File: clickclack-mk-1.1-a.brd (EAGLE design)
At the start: 101.6 x 25.4 mm, 23 parts, among them SW1 CHERRY-MXNONUBS, SW2 CHERRY-MXNONUBS, SW3 CHERRY-MXNONUBS, SW4 CHERRY-MXNONUBS, SW5 CHERRY-MXNONUBS, SW6 CHERRY-MXNONUBS, U1 TEENSY_3.0_BASIC_ALTDIP

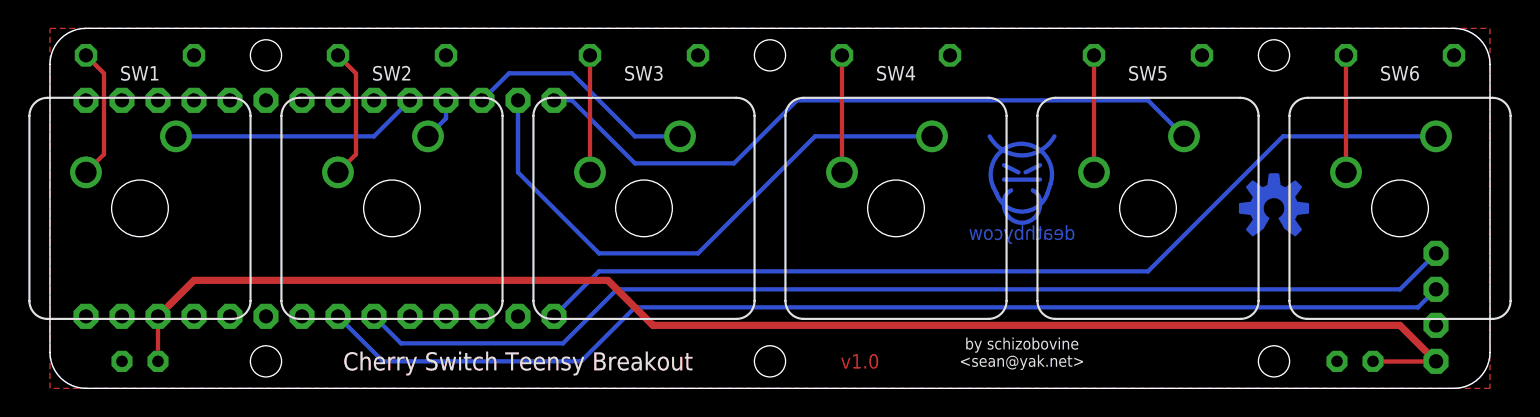
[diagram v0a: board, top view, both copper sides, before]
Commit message: [wip] do not use
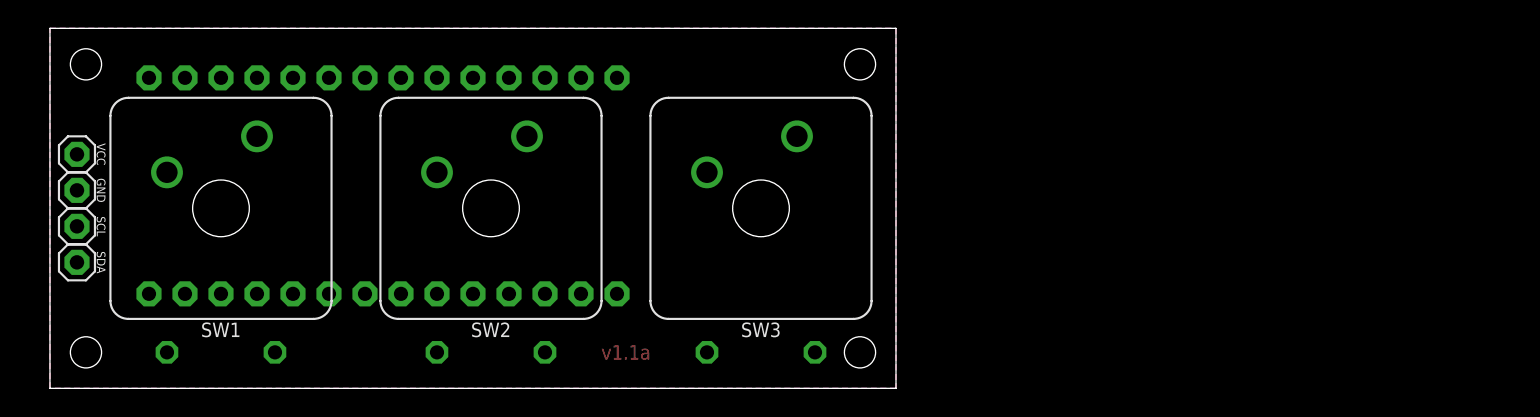
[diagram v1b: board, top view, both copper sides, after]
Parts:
- removed C1, C2: 100n, A_butts:C025-024X044
- removed D4, D5, D6: 1N4148, A_butts:DIODE-7.62MM
- removed SW4, SW5, SW6: CHERRY-MXNONUBS, A_butts:CHERRY-MX-NONUBS
- removed U$1: (no value), A_butts:CC-BY-SA-4.0-URL-BOTTOM
- removed U$3: (no value), A_butts:COW_SMALL_METAL
- removed U$4: (no value), A_butts:OSHWLOGO_5MM_METAL
- moved VCC 97.0 mm to (1.91, 16.5), flipped to the top
- moved GND 96.4 mm to (1.91, 14.0), flipped to the top
- moved SCL 96.0 mm to (1.91, 11.4), flipped to the top
- moved SDA 95.9 mm to (1.91, 8.89), flipped to the top
- moved D3 22.5 mm to (50.2, 2.54)
- moved D2 22.1 mm to (31.1, 2.54)
- moved D1 21.7 mm to (12.1, 2.54)
- moved SW3 8.26 mm to (50.2, 12.7)
- moved SW2 6.98 mm to (31.1, 12.7)
- moved SW1 5.71 mm to (12.1, 12.7)
- moved U1 4.72 mm to (23.5, 14.3)
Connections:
- removed net N$4: D4.A, SW4.1
- removed net N$5: D5.A, SW5.1
- removed net N$6: D6.A, SW6.1
- net GND: no longer C1.2, C2.2, D4.K, D5.K, D6.K
- net KEY4: no longer SW4.2
- net KEY5: no longer SW5.2
- net KEY6: no longer SW6.2
- net VCC: no longer C1.1, C2.1
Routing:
- net VCC: track 101.2 -> 0.00 mm
- net SCL: track 80.9 -> 0.00 mm
- net SDA: track 78.3 -> 0.00 mm
- net KEY6: track 67.5 -> 0.00 mm
- net KEY5: track 49.2 -> 0.00 mm
- net KEY4: track 40.1 -> 0.00 mm
- net KEY1: track 17.6 -> 0.00 mm
- net KEY3: track 16.6 -> 0.00 mm
- net N$2: track 9.31 -> 0.00 mm
- net N$1: track 9.31 -> 0.00 mm
- net N$6: track 8.26 -> 0.00 mm
- net N$5: track 8.26 -> 0.00 mm
- net N$4: track 8.26 -> 0.00 mm
- net N$3: track 8.26 -> 0.00 mm
- net KEY2: track 3.07 -> 0.00 mm
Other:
- board size 101.6 x 25.4 mm -> 59.7 x 25.4 mm
- board text removed: "Cherry Switch Teensy Breakout"
- board text removed: "by schizobovine <sean@yak.net>"
